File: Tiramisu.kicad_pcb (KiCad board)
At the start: 2 copper layers, 24 x 32 mm, 26 parts, among them J1 Conn_ARM_SWD_TagConnect_TC203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, J2 USB_C_Receptacle_USB2.0_16P, Q1 Q_PMOS_GSD, U1 MDBT50Q-1MV2, U2 LSM6DSV, U3 MCP73831-2-OT

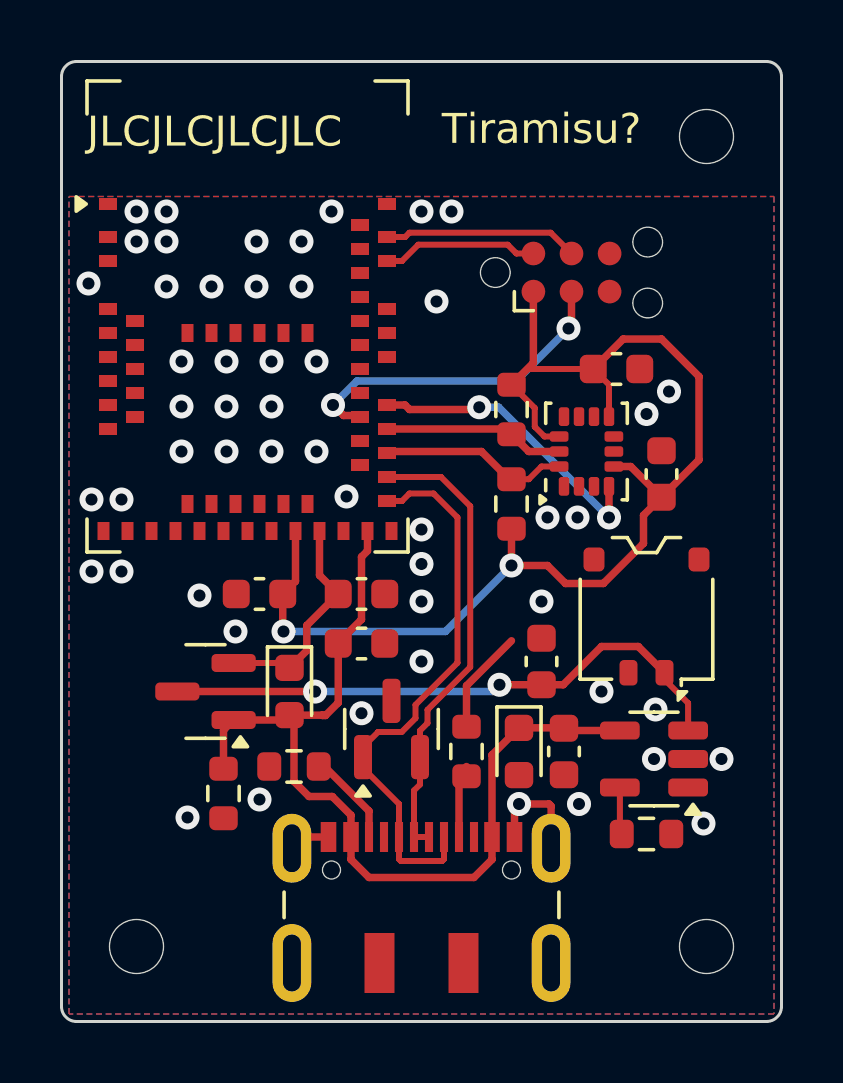
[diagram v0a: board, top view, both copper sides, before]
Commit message: final export
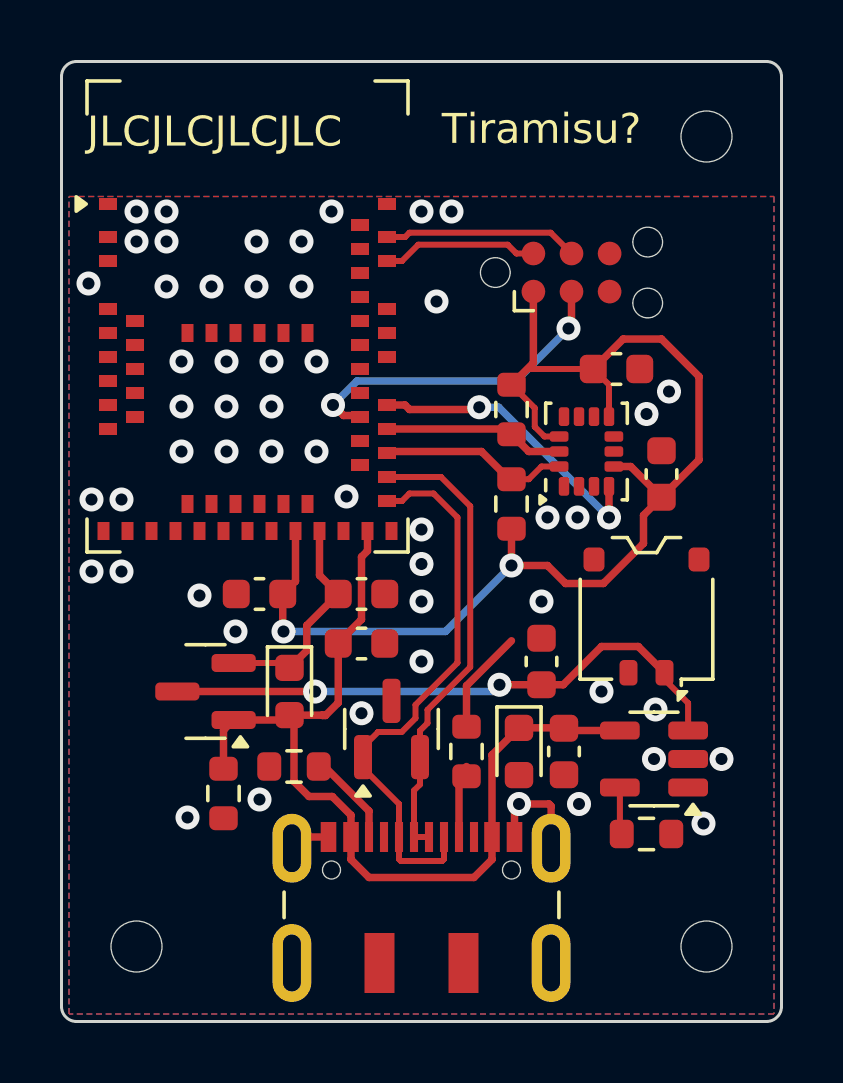
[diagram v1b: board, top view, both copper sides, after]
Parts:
- H1, H2, H3: footprint adhoc:MountingHole_1.8mm_M1.6 -> adhoc:MountingHole_1.7mm_M1.6
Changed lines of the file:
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@@
 			(plot_on_all_layers_selection 0x0000000_00000000)
 			(disableapertmacros no)
-			(usegerberextensions no)
-			(usegerberattributes yes)
-			(usegerberadvancedattributes yes)
-			(creategerberjobfile yes)
+			(usegerberextensions yes)
+			(usegerberattributes no)
+			(usegerberadvancedattributes no)
+			(creategerberjobfile no)
 			(dashed_line_dash_ratio 12.000000)
 			(dashed_line_gap_ratio 3.000000)
@@
 			(plotinvisibletext no)
 			(sketchpadsonfab no)
-			(subtractmaskfromsilk no)
+			(subtractmaskfromsilk yes)
 			(outputformat 1)
 			(mirror no)
-			(drillshape 1)
+			(drillshape 0)
 			(scaleselection 1)
-			(outputdirectory "")
+			(outputdirectory "gerbers/")
 		)
 	)
@@
 		)
 	)
-	(footprint "adhoc:MountingHole_1.8mm_M1.6"
+	(footprint "adhoc:MountingHole_1.7mm_M1.6"
 		(layer "F.Cu")
 		(at 121.5 79.5)
@@
 			)
 		)
-		(property "Footprint" "adhoc:MountingHole_1.8mm_M1.6"
+		(property "Footprint" "adhoc:MountingHole_1.7mm_M1.6"
 			(at 0 0 0)
 			(unlocked yes)
@@
 		(pad "" np_thru_hole circle
 			(at 0 0)
-			(size 1.8 1.8)
-			(drill 1.8)
-			(layers "F&B.Cu" "*.Mask")
+			(size 1.7 1.7)
+			(drill 1.7)
+			(layers "F&B.Cu" "*.Paste" "*.Mask")
 		)
 	)
@@
 		)
 	)
-	(footprint "adhoc:MountingHole_1.8mm_M1.6"
+	(footprint "adhoc:MountingHole_1.7mm_M1.6"
 		(layer "F.Cu")
 		(at 121.5 52.5)
@@
 			)
 		)
-		(property "Footprint" "adhoc:MountingHole_1.8mm_M1.6"
+		(property "Footprint" "adhoc:MountingHole_1.7mm_M1.6"
 			(at 0 0 0)
 			(unlocked yes)
@@
 		(pad "" np_thru_hole circle
 			(at 0 0)
-			(size 1.8 1.8)
-			(drill 1.8)
-			(layers "F&B.Cu" "*.Mask")
+			(size 1.7 1.7)
+			(drill 1.7)
+			(layers "F&B.Cu" "*.Paste" "*.Mask")
 		)
 	)
@@
 		)
 	)
-	(footprint "adhoc:MountingHole_1.8mm_M1.6"
+	(footprint "adhoc:MountingHole_1.7mm_M1.6"
 		(layer "F.Cu")
 		(at 102.5 79.5)
@@
 			)
 		)
-		(property "Footprint" "adhoc:MountingHole_1.8mm_M1.6"
+		(property "Footprint" "adhoc:MountingHole_1.7mm_M1.6"
 			(at 0 0 0)
 			(unlocked yes)
@@
 		(pad "" np_thru_hole circle
 			(at 0 0)
-			(size 1.8 1.8)
-			(drill 1.8)
-			(layers "F&B.Cu" "*.Mask")
+			(size 1.7 1.7)
+			(drill 1.7)
+			(layers "F&B.Cu" "*.Paste" "*.Mask")
 		)
 	)
